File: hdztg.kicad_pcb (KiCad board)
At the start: 4 copper layers, 37 x 18 mm, 8 parts, among them J1 20374-R20E-31, Q1 2N7002KDW 72K

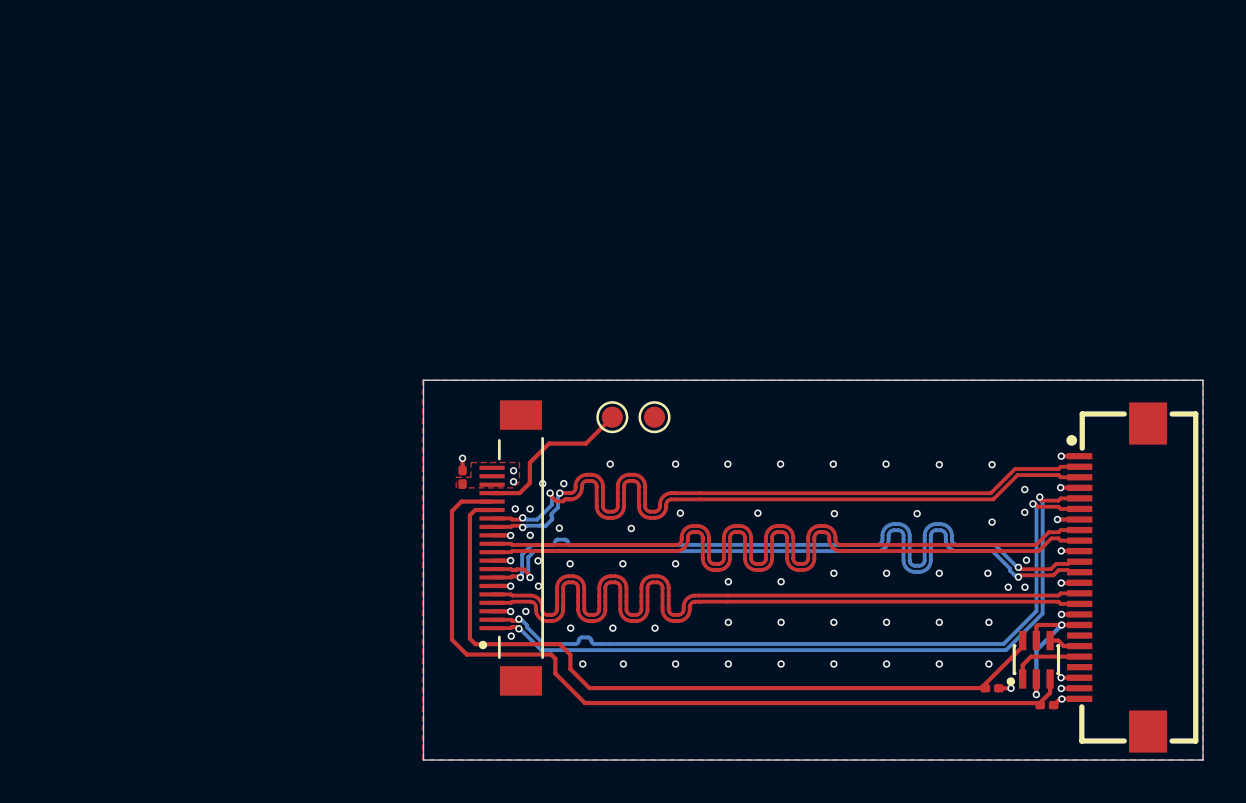
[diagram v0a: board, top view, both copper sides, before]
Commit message: prod
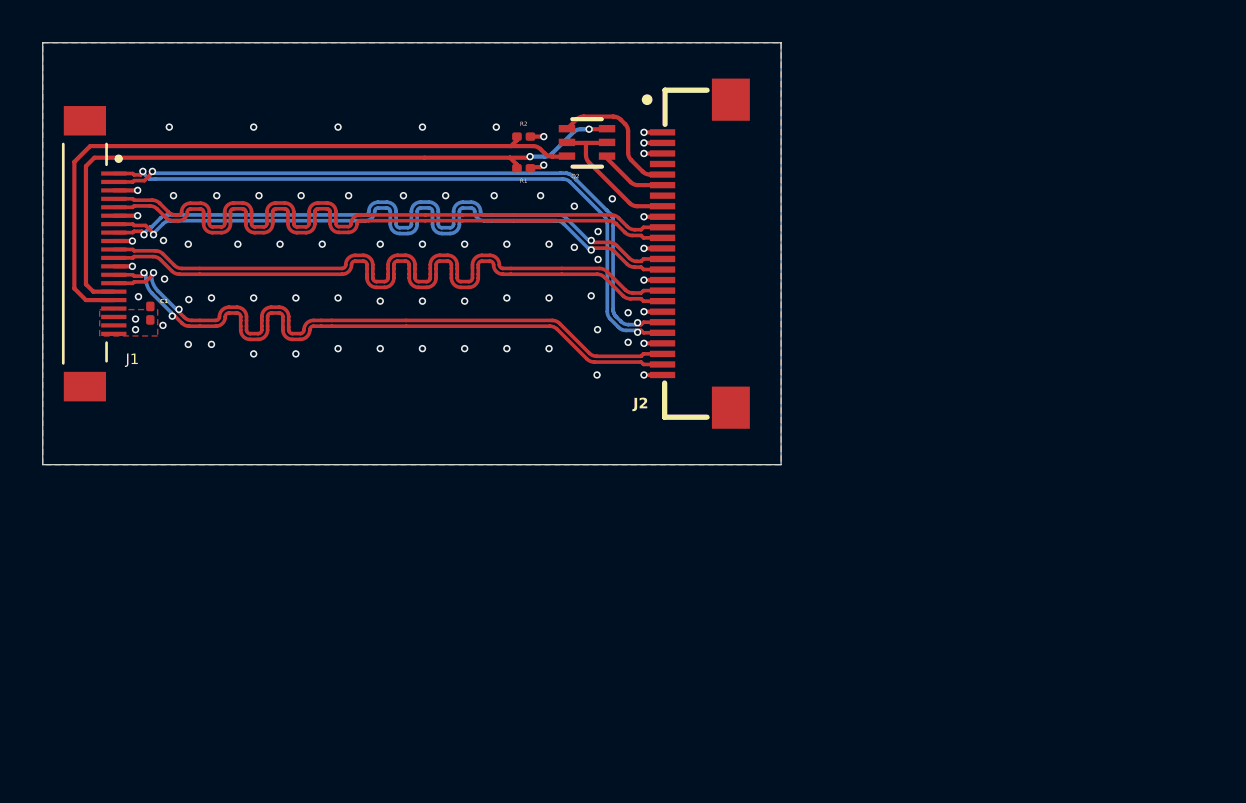
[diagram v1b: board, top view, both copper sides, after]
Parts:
- removed FPC1: FPC-05FB-24PH20, EasyEDA:FPC-SMD_24P-P0.50_FPC-05FB-24PH20
- removed Q1: 2N7002KDW 72K, EasyEDA:SOT-363_L2.1-W1.3-P0.65-LS2.3-BL
- removed TP1, TP2: TestPoint, TestPoint:TestPoint_Pad_D1.0mm
- added J2: FPC-05FB-24PH20, EasyEDA:FPC-SMD_24P-P0.50_FPC-05FB-24PH20, F.Cu at (111.0, 70.0)
- added Q2: BSS138DW-7-F, EasyEDA:SC-70-6_L2.2-W1.3-P0.65-LS2.1-TL, F.Cu at (105.8, 64.7)
- moved R2 36.6 mm to (102.8, 64.5)
- moved R1 33.2 mm to (102.8, 66.0), turned to 0 degrees
- moved J1 24.9 mm to (82.0, 70.0), turned to -90 degrees
- moved C1 16.7 mm to (85.1, 72.8)
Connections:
- R1 pad 1: +3V3 -> /SCL_3V3
- R1 pad 2: /SCL_3V3 -> +3V3
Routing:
- net /PROG: track 7.75 -> 0.00 mm
- net /SDA_3V3: track 39.0 -> 32.5 mm
- net /MIPI_D3+: track 37.7 -> 33.2 mm
- net /MIPI_D3-: track 37.7 -> 33.2 mm
- net /MIPI_CK-: track 37.7 -> 33.2 mm
- net /MIPI_CK+: track 37.7 -> 33.2 mm
- net /SCL_1V8: track 3.53 -> 6.64 mm
- net /MIPI_D1-: track 34.8 -> 31.8 mm
- net /MIPI_D1+: track 34.8 -> 31.9 mm
- net /MIPI_D0-: track 34.9 -> 32.0 mm
- net /MIPI_D0+: track 34.9 -> 32.0 mm
- net /SCL_3V3: track 35.7 -> 33.0 mm, vias 0 -> 2
- net /MIPI_D2+: track 34.5 -> 31.8 mm
- net /MIPI_D2-: track 34.5 -> 31.8 mm
- net /SDA_1V8: track 1.51 -> 3.26 mm
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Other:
- board size 37 x 18 mm -> 35 x 20 mm
